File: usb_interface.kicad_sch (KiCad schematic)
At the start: 14 parts, among them J15 USB_C_Receptacle, U2 TPS25730D, U4 TVS2200DRV

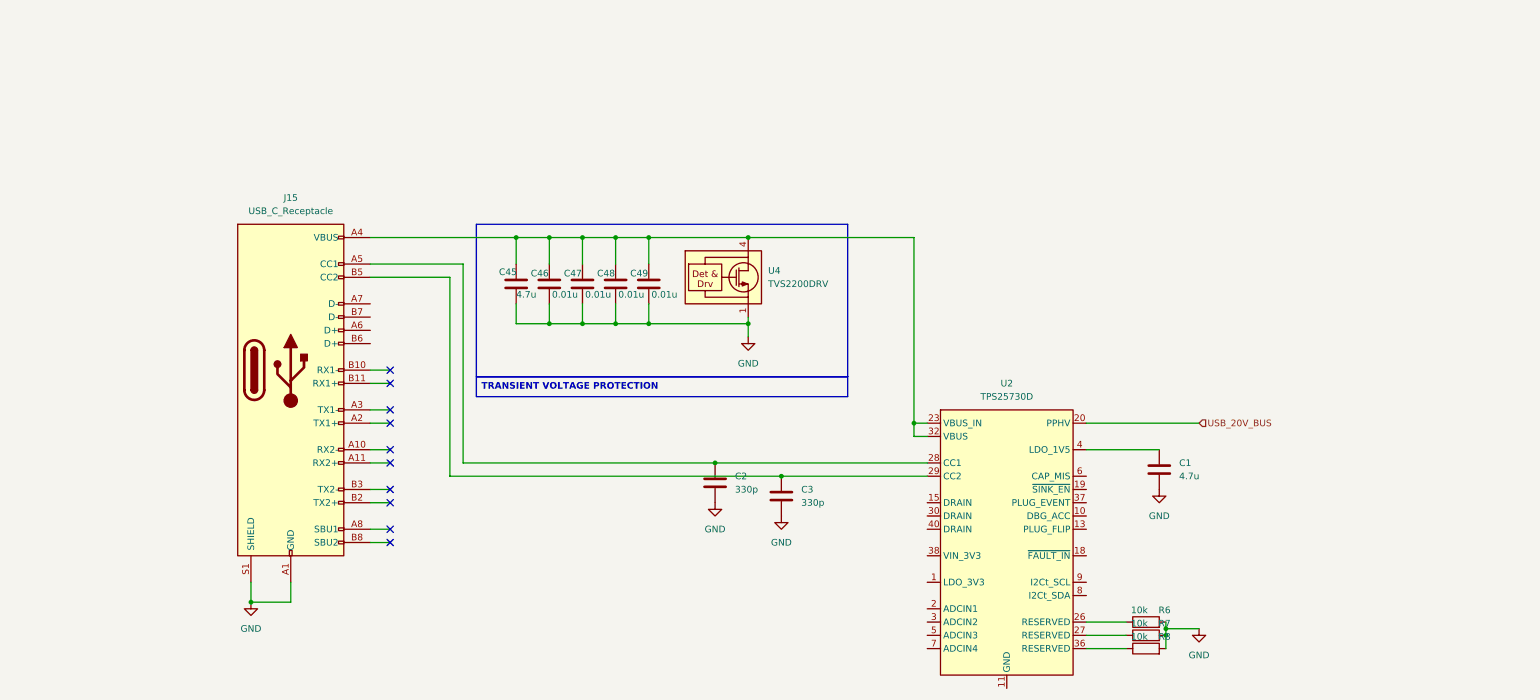
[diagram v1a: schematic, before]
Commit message: structural changes
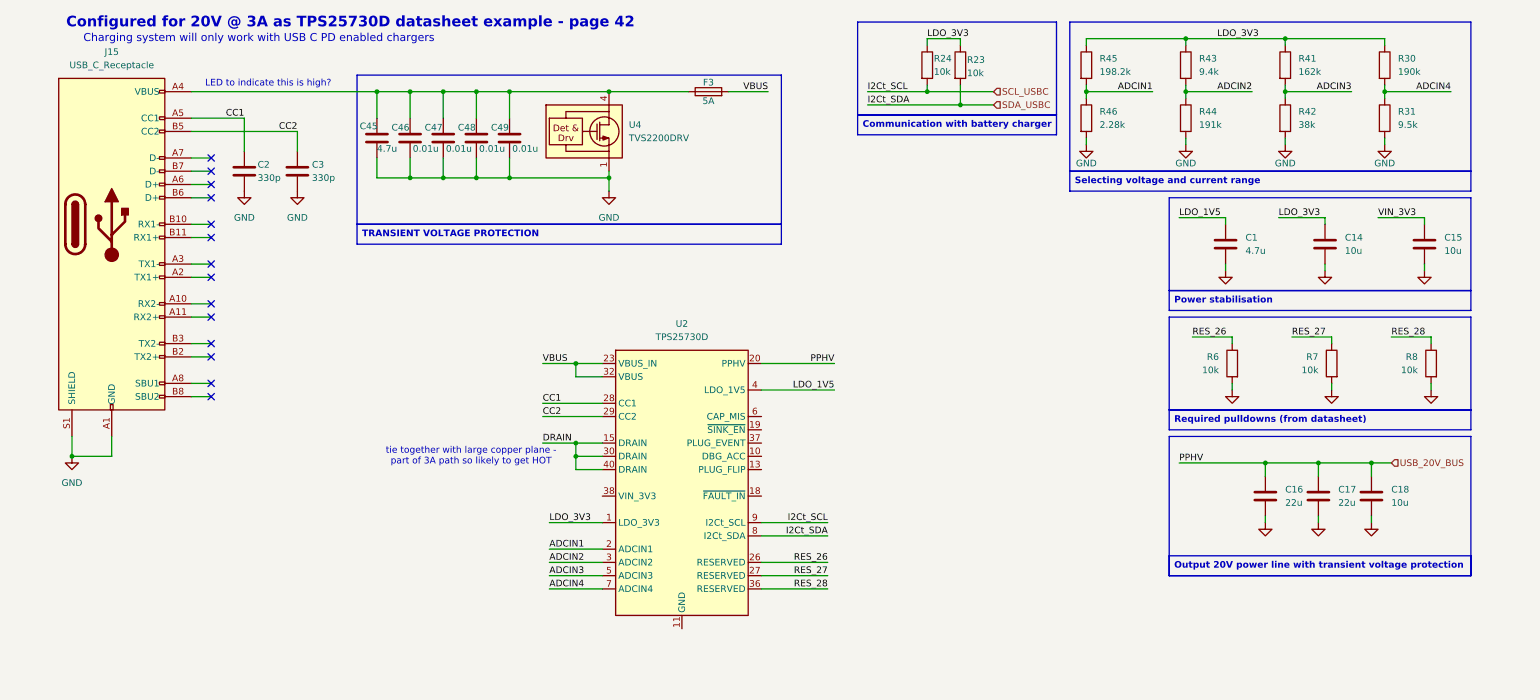
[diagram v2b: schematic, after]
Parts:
- added C14, C15, C18: 10u, symbol Device:C
- added C16, C17: 22u, symbol Device:C
- added F3: 5A, symbol Device:Fuse
- added R23, R24: 10k, symbol Device:R
- added R30: 190k, symbol Device:R
- added R31: 9.5k, symbol Device:R
- added R41: 162k, symbol Device:R
- added R42: 38k, symbol Device:R
- added R43: 9.4k, symbol Device:R
- added R44: 191k, symbol Device:R
- added R45: 198.2k, symbol Device:R
- added R46: 2.28k, symbol Device:R
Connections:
- net GND: now also C14.2, C15.2, C16.2, C17.2, C18.2, R31.2, R42.2, R44.2, R46.2
- net USB_20V_BUS: now also C16.1, C17.1, C18.1
- net CC1: now reaches C2.1, J15.A5 (CC1), U2.28 (CC1)
- net RES_26: now reaches R6.1, U2.26 (RESERVED)
- net at C45.1, C46.1, C47.1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: now also F3.1; no longer U2.23 (VBUS_IN), U2.32 (VBUS)
- net RES_28: now reaches R8.1, U2.36 (RESERVED)
- net LDO_3V3: now reaches U2.1 (LDO_3V3)
- net LDO_3V3: now also C14.1, R23.1, R24.1, R30.1, R41.1, R43.1, R45.1
- net DRAIN: now reaches U2.15 (DRAIN)
- net DRAIN: now also U2.30 (DRAIN), U2.40 (DRAIN)
- net ADCIN1: now reaches U2.2 (ADCIN1)
- net ADCIN1: now also R45.2, R46.1
- net RES_27: now reaches R7.1, U2.27 (RESERVED)
- net CC2: now reaches C3.1, J15.B5 (CC2), U2.29 (CC2)
- net ADCIN2: now reaches U2.3 (ADCIN2)
- net ADCIN2: now also R43.2, R44.1
- net LDO_1V5: now reaches C1.1, U2.4 (LDO_1V5)
- net ADCIN3: now reaches U2.5 (ADCIN3)
- net ADCIN3: now also R41.2, R42.1
- net ADCIN4: now reaches U2.7 (ADCIN4)
- net ADCIN4: now also R30.2, R31.1
- net SDA_USBC: now reaches U2.8 (I2Ct_SDA)
- net SDA_USBC: now also R23.2
- net SCL_USBC: now reaches U2.9 (I2Ct_SCL)
- net SCL_USBC: now also R24.2
- new net VBUS: F3.2, U2.23 (VBUS_IN), U2.32 (VBUS)
- new net VIN_3V3: C15.1
- no-connect marks 10 -> 14
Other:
- note added: "Charging system will only work with USB C PD enabled chargers"
- note added: "Configured for 20V @ 3A as TPS25730D datasheet example - page 42"
- note added: "LED to indicate this is high?"
- note added: "tie together with large copper plane - part of 3A path so likely to get HOT"
- moved on the sheet: C1, C2, C3, C45, C46, C47, C48, C49, J15, U2, U4
